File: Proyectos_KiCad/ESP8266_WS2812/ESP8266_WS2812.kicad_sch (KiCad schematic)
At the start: 15 parts, among them J1 LOAD, J3 HOME, J4 V_WS2812, J5 WS2812, J6 AC_VIN, Q1 BT136-800, U1 MOC3021M

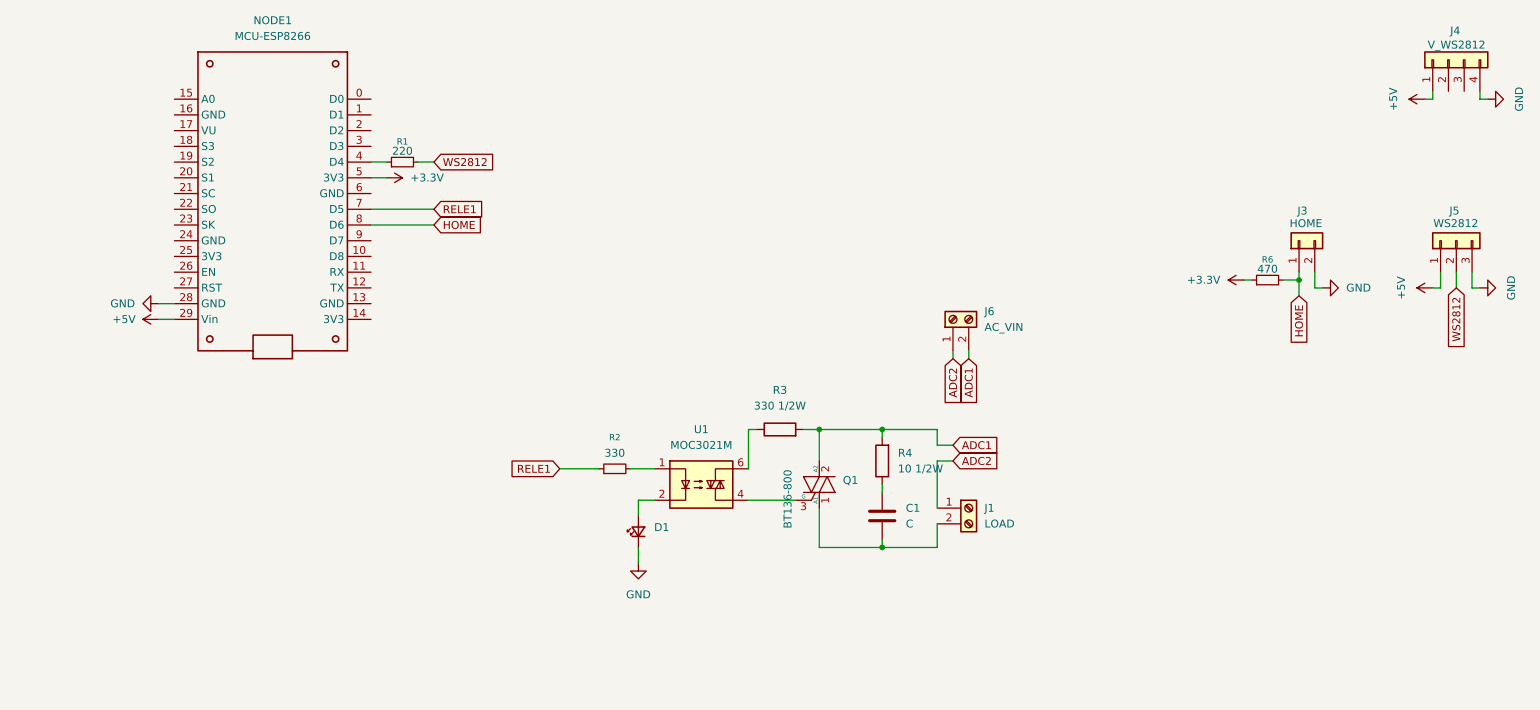
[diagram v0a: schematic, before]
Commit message: Omarchy-RIP
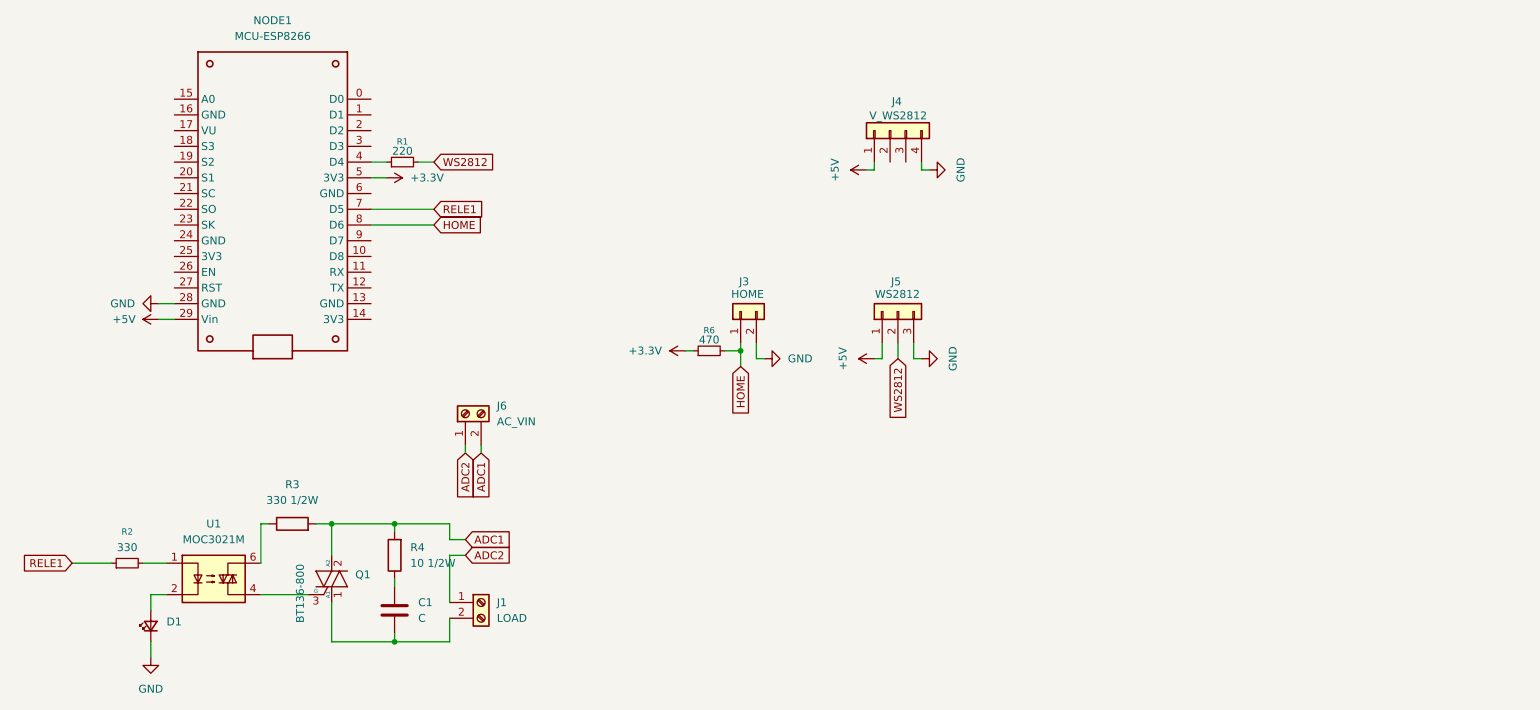
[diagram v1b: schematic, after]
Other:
- moved on the sheet: C1, D1, J1, J3, J4, J5, J6, Q1, R2, R3, R4, R6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
